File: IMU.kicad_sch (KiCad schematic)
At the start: 0 parts

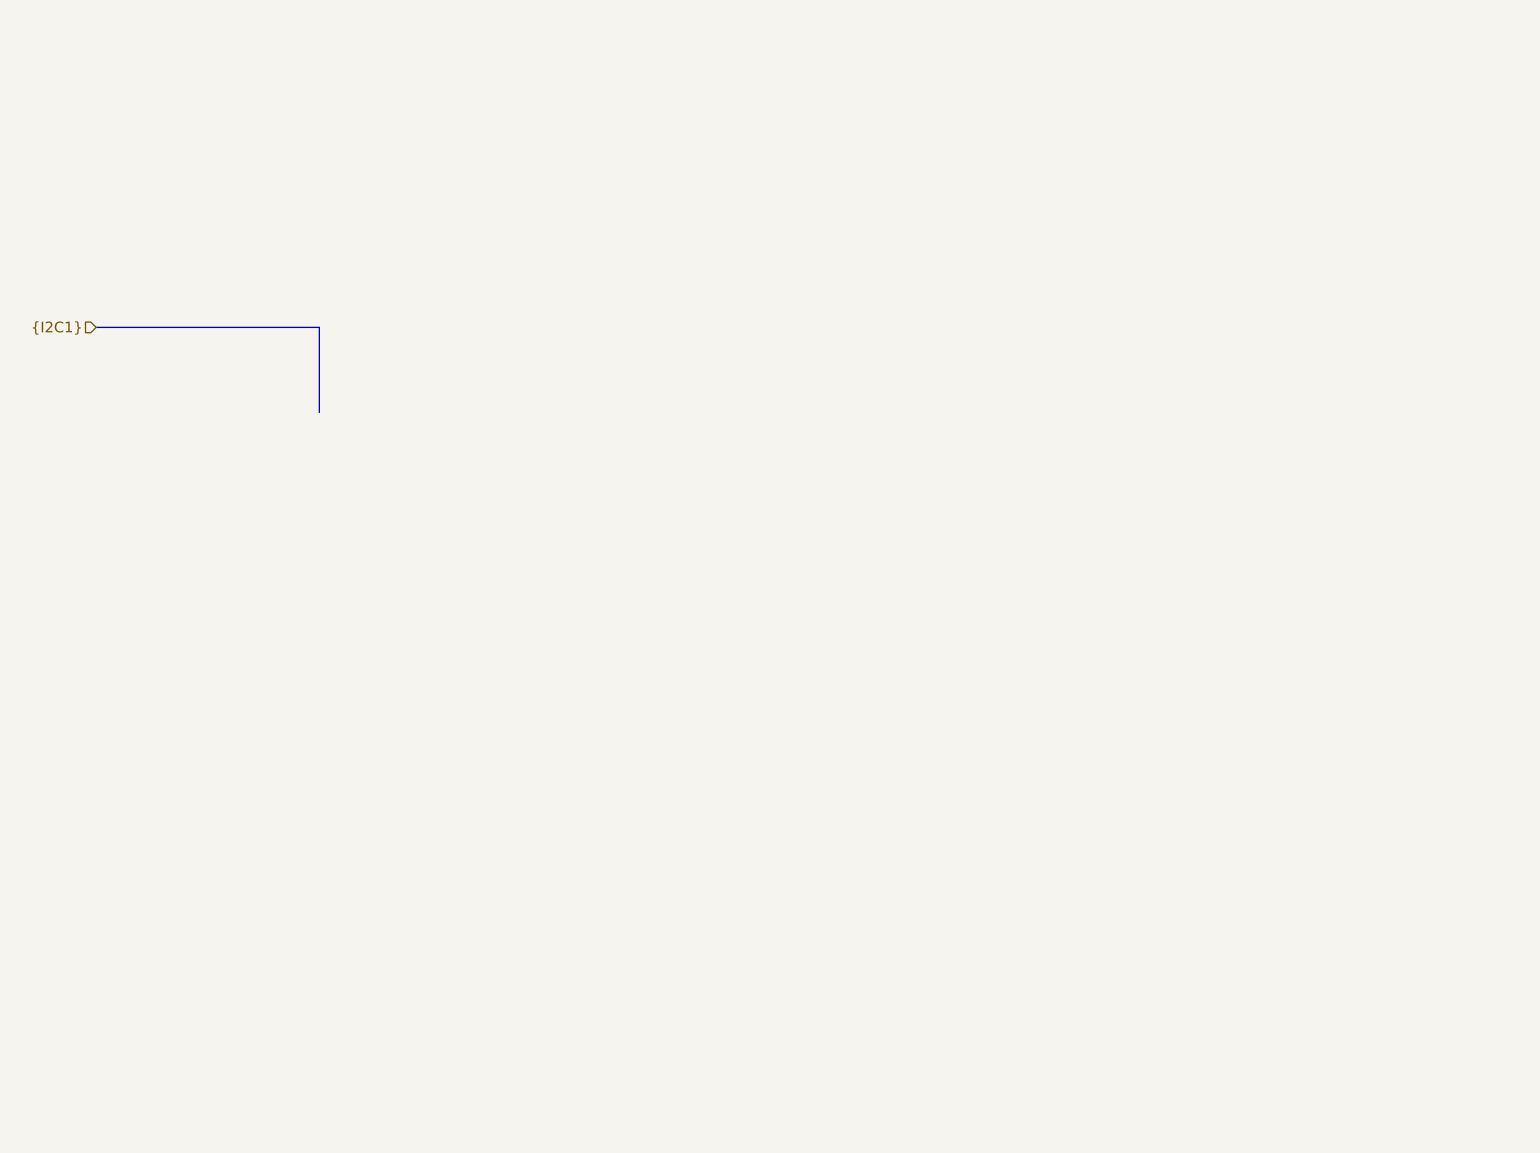
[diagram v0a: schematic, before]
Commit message: IMU block implementation
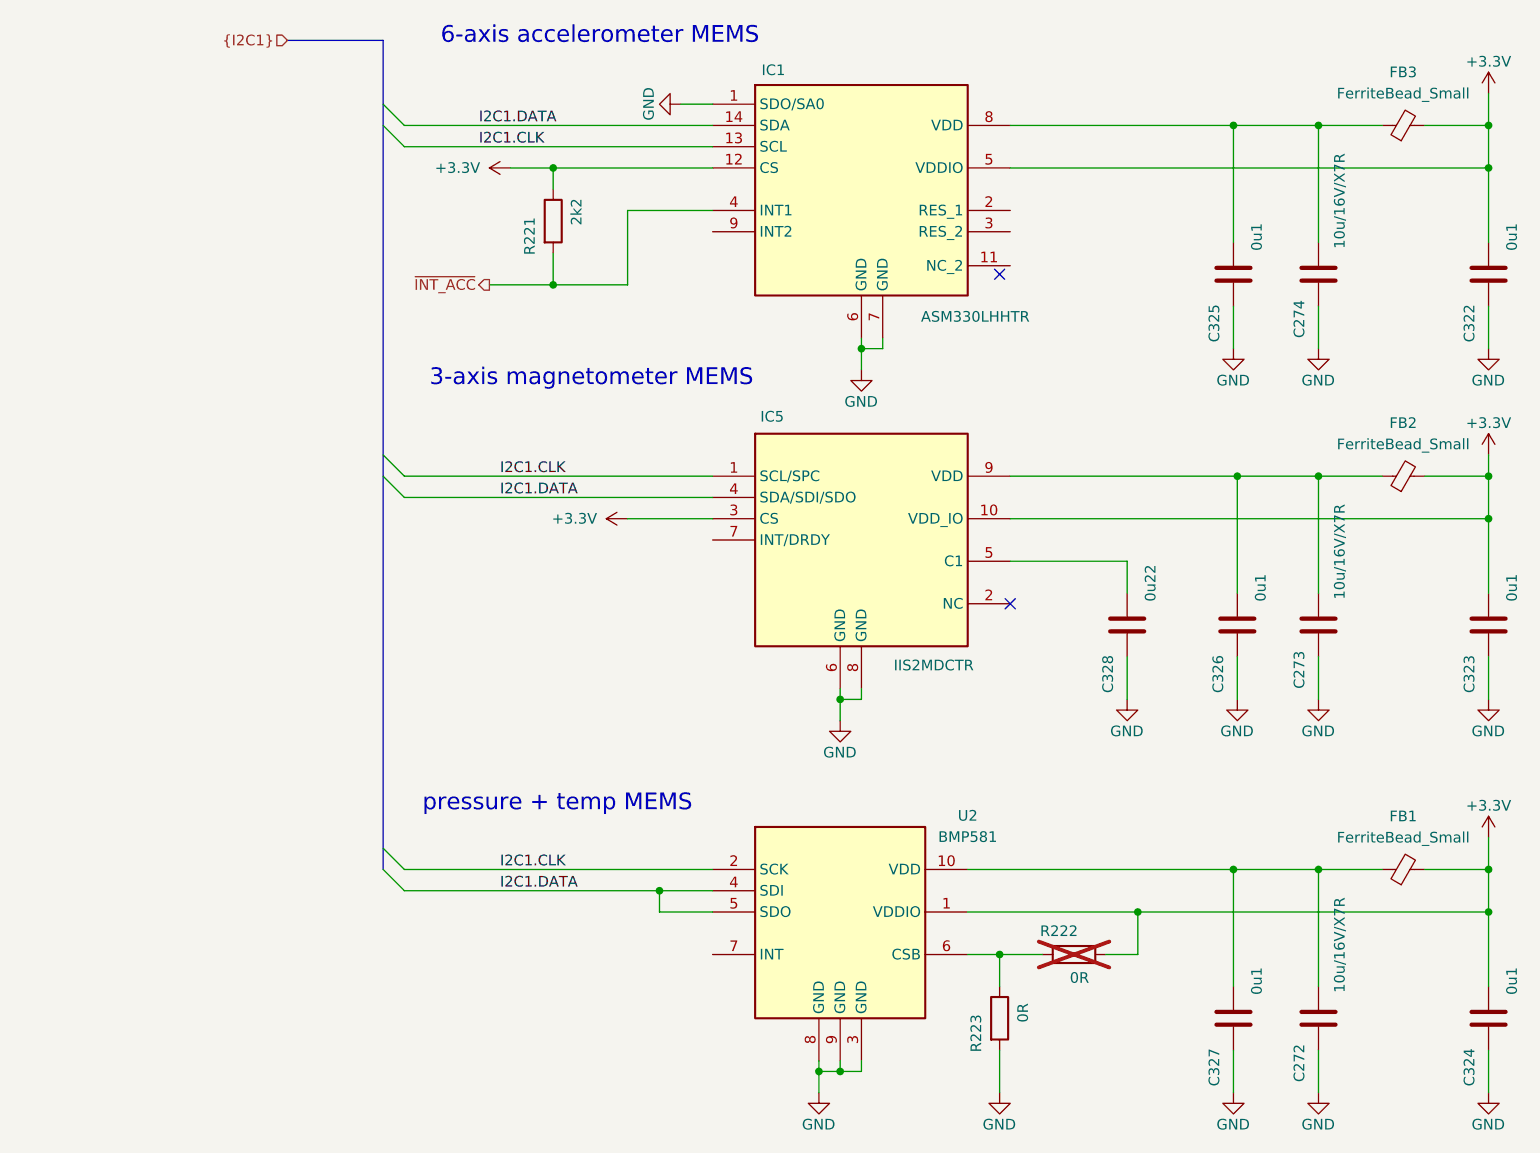
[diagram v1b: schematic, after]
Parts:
- added C272, C273, C274: 10u/16V/X7R, Capacitor_SMD:C_0805_2012Metric, symbol Device:C
- added C322, C323, C324, C325, C326, C327: 0u1, Capacitor_SMD:C_0603_1608Metric, symbol Device:C
- added C328: 0u22, Capacitor_SMD:C_0603_1608Metric, symbol Device:C
- added FB1, FB2, FB3: FerriteBead_Small, Inductor_SMD:L_0603_1608Metric, symbol Device:FerriteBead_Small
- added IC1: ASM330LHHTR, LSM6DS3USTR, symbol E-M-IntegratedCircuits:ASM330LHHTR
- added IC5: IIS2MDCTR, IIS2MDCTR, symbol E-M-IntegratedCircuits:IIS2MDCTR
- added R221: 2k2, Resistor_SMD:R_0603_1608Metric, symbol Device:R
- added R222, R223: 0R, Resistor_SMD:R_0603_1608Metric, symbol Device:R
- added U2: BMP581, BMP581, symbol E-M-IntegratedCircuits:BMP581
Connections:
- new net: R222.2, R223.1, U2.6 (CSB)
- new net: C273.1, C326.1, FB2.1, IC5.9 (VDD)
- new net: C328.1, IC5.5 (C1)
- new net: C274.1, C325.1, FB3.1, IC1.8 (VDD)
- new net: C272.1, C327.1, FB1.1, U2.10 (VDD)
- new net: IC1.10 (NC_1), IC1.11 (NC_2)
- new net: IC5.11 (NC), IC5.12 (NC), IC5.2 (NC)
- new net +3.3V: C322.1, C323.1, C324.1, FB1.2, FB2.2, FB3.2, IC1.12 (CS), IC1.5 (VDDIO), IC5.10 (VDD_IO), IC5.3 (CS), R221.1, R222.1, U2.1 (VDDIO)
- new net GND: C272.2, C273.2, C274.2, C322.2, C323.2, C324.2, C325.2, C326.2, C327.2, C328.2, IC1.1 (SDO/SA0), IC1.6 (GND), IC1.7 (GND), IC5.6 (GND), IC5.8 (GND), R223.2, U2.3 (GND), U2.8 (GND), U2.9 (GND)
- new net I2C1.CLK: IC1.13 (SCL), IC5.1 (SCL/SPC), U2.2 (SCK)
- new net I2C1.DATA: IC1.14 (SDA), IC5.4 (SDA/SDI/SDO), U2.4 (SDI), U2.5 (SDO)
- new net ~{INT_ACC}: IC1.4 (INT1), R221.2
- no-connect marks 0 -> 2
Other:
- note added: "3-axis magnetometer MEMS"
- note added: "6-axis accelerometer MEMS"
- note added: "pressure + temp MEMS"

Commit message: EMI/EMC meassures implementation + VCU panel interface block
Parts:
- C272, C273, C274, C322, C323, C324, C325, C326, C327, C328: symbol Device:C -> VELION_VCU_Library:C
- FB1, FB2, FB3: symbol Device:FerriteBead_Small -> VELION_VCU_Library:FerriteBead_Small
- IC1: footprint LSM6DS3USTR -> E-M-IntegratedCircuits:LSM6DS3USTR; symbol E-M-IntegratedCircuits:ASM330LHHTR -> VELION_VCU_Library:ASM330LHHTR
- IC5: footprint IIS2MDCTR -> E-M-IntegratedCircuits:IIS2MDCTR; symbol E-M-IntegratedCircuits:IIS2MDCTR -> VELION_VCU_Library:IIS2MDCTR
- R221, R222, R223: symbol Device:R -> VELION_VCU_Library:R
- U2: footprint BMP581 -> E-M-IntegratedCircuits:BMP581; symbol E-M-IntegratedCircuits:BMP581 -> VELION_VCU_Library:BMP581
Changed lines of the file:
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@@
 	)
 	(symbol
-		(lib_id "Device:R")
+		(lib_id "VELION_VCU_Library:R")
 		(at 152.4 137.16 0)
 		(unit 1)
@@
 	)
 	(symbol
-		(lib_id "Device:C")
+		(lib_id "VELION_VCU_Library:C")
 		(at 190.5 90.17 0)
 		(unit 1)
@@
 	)
 	(symbol
-		(lib_id "Device:R")
+		(lib_id "VELION_VCU_Library:R")
 		(at 161.29 129.54 270)
 		(unit 1)
@@
 	)
 	(symbol
-		(lib_id "Device:C")
+		(lib_id "VELION_VCU_Library:C")
 		(at 167.64 90.17 0)
 		(unit 1)
@@
 	)
 	(symbol
-		(lib_id "Device:C")
+		(lib_id "VELION_VCU_Library:C")
 		(at 210.82 137.16 0)
 		(unit 1)
@@
 	)
 	(symbol
-		(lib_id "Device:FerriteBead_Small")
+		(lib_id "VELION_VCU_Library:FerriteBead_Small")
 		(at 200.66 30.48 90)
 		(unit 1)
@@
 	)
 	(symbol
-		(lib_id "Device:C")
+		(lib_id "VELION_VCU_Library:C")
 		(at 180.34 137.16 0)
 		(unit 1)
@@
 	)
 	(symbol
-		(lib_id "Device:C")
+		(lib_id "VELION_VCU_Library:C")
 		(at 180.34 48.26 0)
 		(unit 1)
@@
 	)
 	(symbol
-		(lib_id "Device:FerriteBead_Small")
+		(lib_id "VELION_VCU_Library:FerriteBead_Small")
 		(at 200.66 72.39 90)
 		(unit 1)
@@
 	)
 	(symbol
-		(lib_id "Device:C")
+		(lib_id "VELION_VCU_Library:C")
 		(at 190.5 137.16 0)
 		(unit 1)
@@
 	)
 	(symbol
-		(lib_id "Device:C")
+		(lib_id "VELION_VCU_Library:C")
 		(at 210.82 48.26 0)
 		(unit 1)
@@
 	)
 	(symbol
-		(lib_id "E-M-IntegratedCircuits:ASM330LHHTR")
+		(lib_id "VELION_VCU_Library:ASM330LHHTR")
 		(at 118.11 27.94 0)
 		(unit 1)
@@
 			)
 		)
-		(property "Footprint" "LSM6DS3USTR"
+		(property "Footprint" "E-M-IntegratedCircuits:LSM6DS3USTR"
 			(at 149.86 115.24 0)
 			(hide yes)
@@
 	)
 	(symbol
-		(lib_id "E-M-IntegratedCircuits:BMP581")
+		(lib_id "VELION_VCU_Library:BMP581")
 		(at 118.11 119.38 0)
 		(unit 1)
@@
 			)
 		)
-		(property "Footprint" "BMP581"
+		(property "Footprint" "E-M-IntegratedCircuits:BMP581"
 			(at 144.78 204.14 0)
 			(hide yes)
@@
 	)
 	(symbol
-		(lib_id "Device:C")
+		(lib_id "VELION_VCU_Library:C")
 		(at 190.5 48.26 0)
 		(unit 1)
@@
 	)
 	(symbol
-		(lib_id "Device:C")
+		(lib_id "VELION_VCU_Library:C")
 		(at 180.8023 90.17 0)
 		(unit 1)
@@
 	)
 	(symbol
-		(lib_id "Device:R")
+		(lib_id "VELION_VCU_Library:R")
 		(at 99.06 41.91 0)
 		(unit 1)
@@
 	)
 	(symbol
-		(lib_id "E-M-IntegratedCircuits:IIS2MDCTR")
+		(lib_id "VELION_VCU_Library:IIS2MDCTR")
 		(at 118.11 72.39 0)
 		(unit 1)
@@
 			)
 		)
-		(property "Footprint" "IIS2MDCTR"
+		(property "Footprint" "E-M-IntegratedCircuits:IIS2MDCTR"
 			(at 157.48 167.31 0)
 			(hide yes)
@@
 	)
 	(symbol
-		(lib_id "Device:C")
+		(lib_id "VELION_VCU_Library:C")
 		(at 210.82 90.17 0)
 		(unit 1)
@@
 	)
 	(symbol
-		(lib_id "Device:FerriteBead_Small")
+		(lib_id "VELION_VCU_Library:FerriteBead_Small")
 		(at 200.66 119.38 90)
 		(unit 1)
